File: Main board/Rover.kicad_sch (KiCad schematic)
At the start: 11 parts, among them J1 IN, J2 OUT, J3 Barrel_Jack_Switch, J4 MOTOR, J5 MOTOR, J6 MOTOR, J7 MOTOR, SW1 SW_DPDT_x2, U1 RASPBERRY_PI_4B_4GB

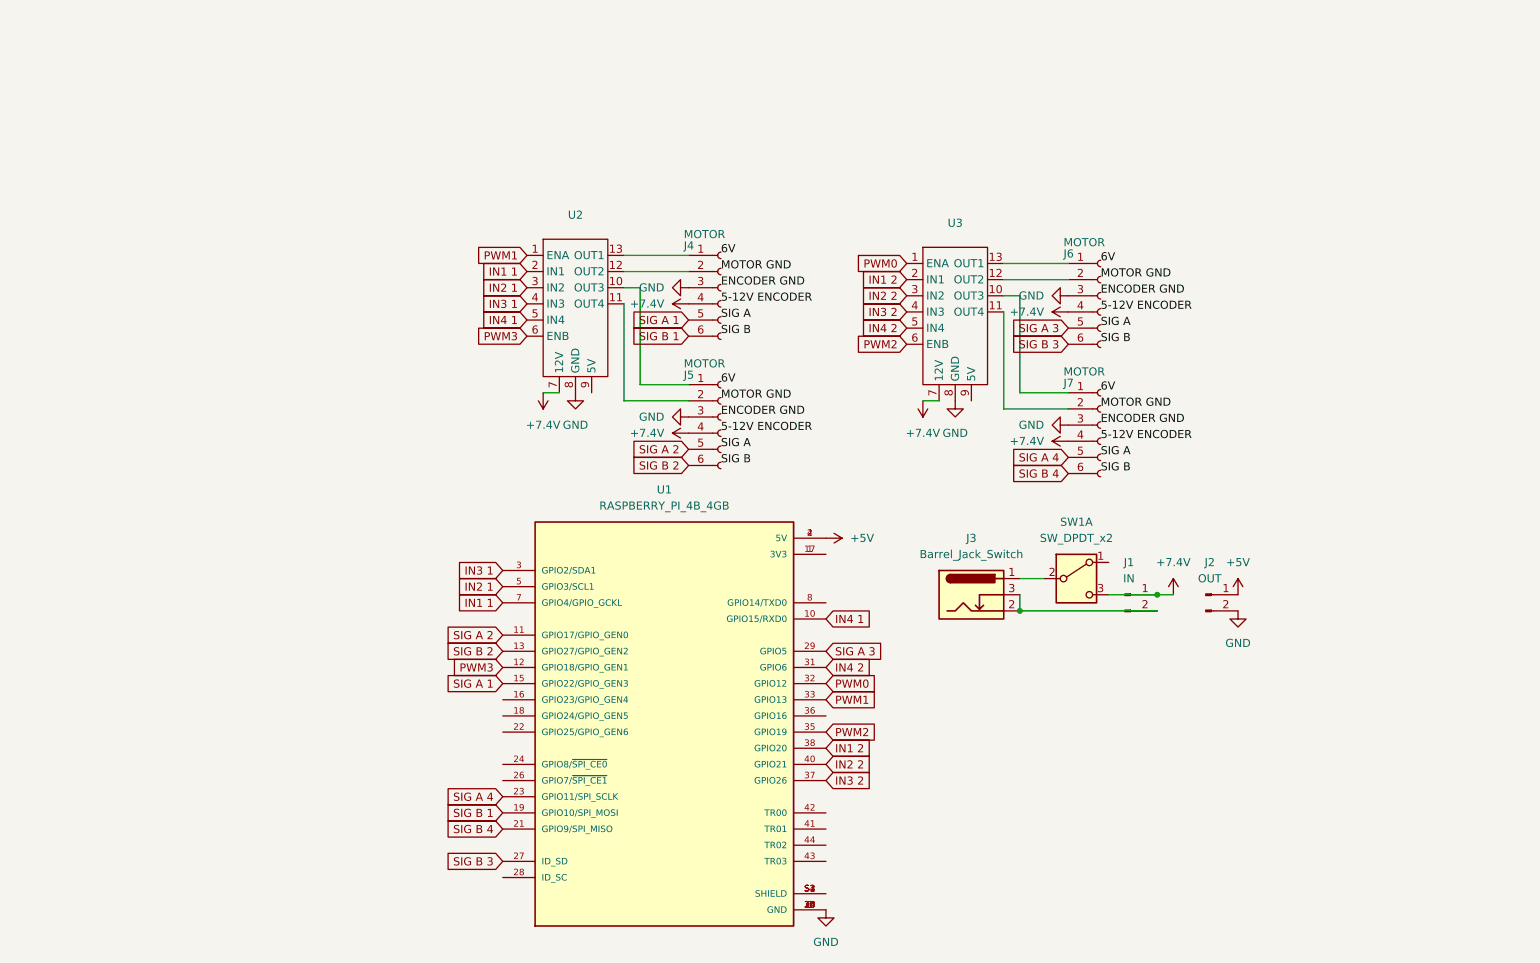
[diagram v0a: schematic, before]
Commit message: updated pcb
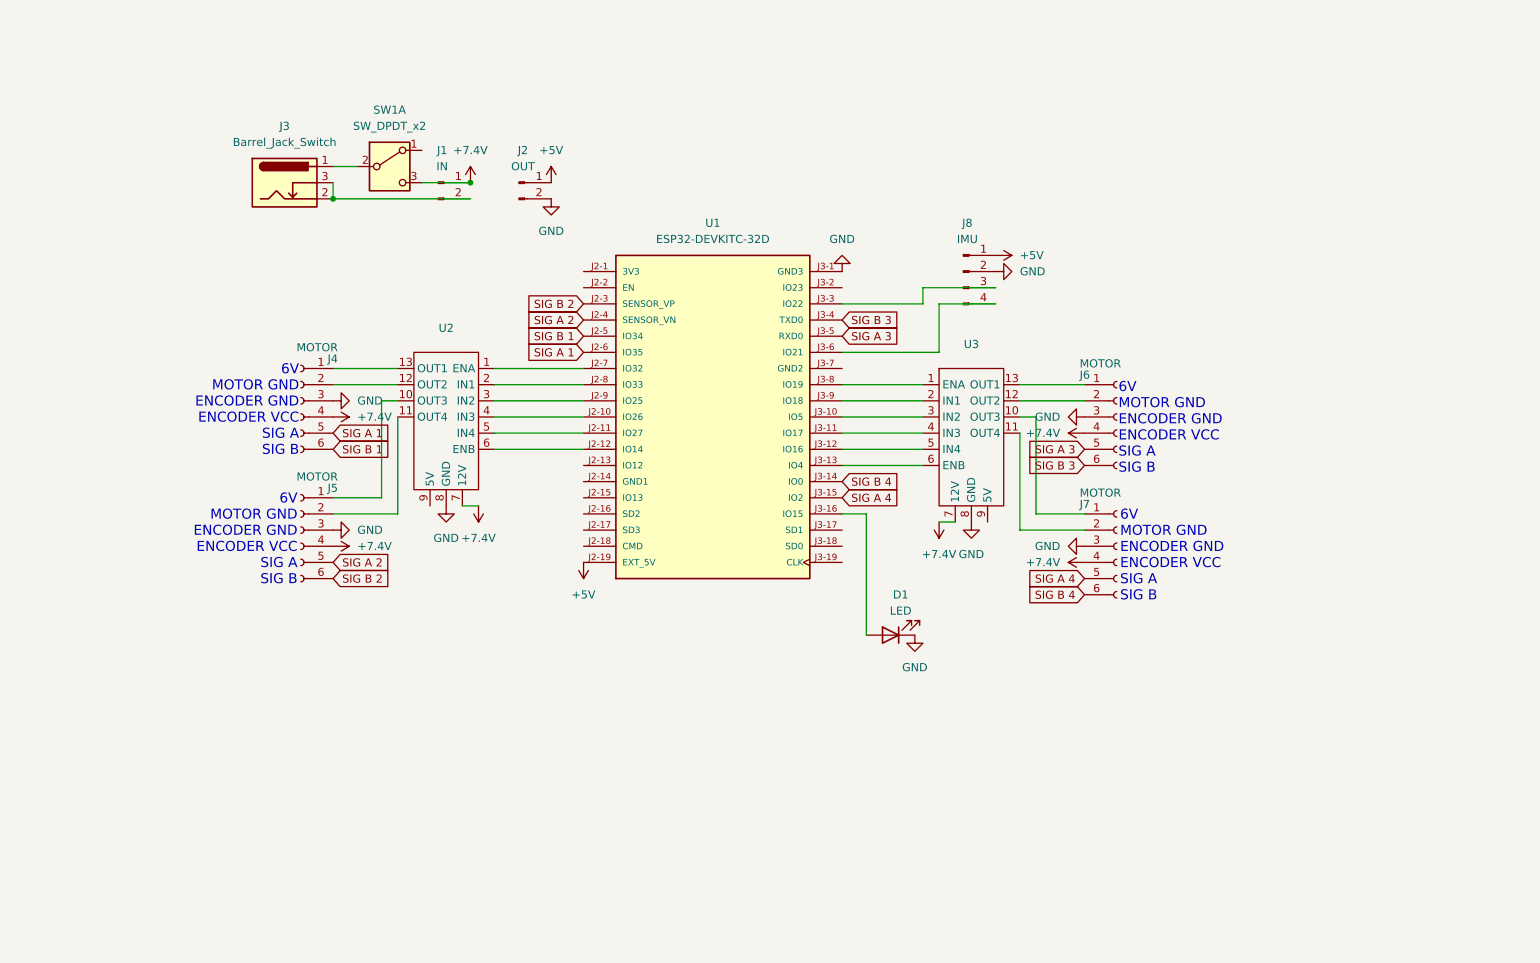
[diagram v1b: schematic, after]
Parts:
- removed U1: RASPBERRY_PI_4B_4GB, RASPBERRY_PI_4B_4GB:MODULE_RASPBERRY_PI_4B_4GB, symbol RASPBERRY_PI_4B_4GB:RASPBERRY_PI_4B_4GB
- added D1: LED, LED_THT:LED_D5.0mm_Clear, symbol Device:LED
- added J8: IMU, Connector_PinHeader_2.54mm:PinHeader_1x08_P2.54mm_Vertical, symbol Connector:Conn_01x04_Pin
- added U1: ESP32-DEVKITC-32D, Library:MODULE_ESP32-DEVKITC-32D, symbol ESP32-DEVKITC-32D:ESP32-DEVKITC-32D
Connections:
- net +5V: now also J8.1 (Pin_1), U1.J2-19 (EXT_5V)
- net GND: now also D1.1 (K), J8.2 (Pin_2), U1.J3-1 (GND3)
- net SIG A 1: now also U1.J2-6 (IO35)
- net SIG A 2: now also U1.J2-4 (SENSOR_VN)
- net SIG A 3: now also U1.J3-5 (RXD0)
- net SIG A 4: now also U1.J3-15 (IO2)
- net SIG B 1: now also U1.J2-5 (IO34)
- net SIG B 2: now also U1.J2-3 (SENSOR_VP)
- net SIG B 3: now also U1.J3-4 (TXD0)
- net SIG B 4: now also U1.J3-14 (IO0)
- net IN1 1: no longer names the net of U2.2 (IN1)
- net IN1 1: now also U1.J2-8 (IO33)
- net IN1 2: no longer names the net of U3.2 (IN1)
- net IN1 2: now also U1.J3-9 (IO18)
- net IN2 1: no longer names the net of U2.3 (IN2)
- net IN2 1: now also U1.J2-9 (IO25)
- net IN2 2: no longer names the net of U3.3 (IN2)
- net IN2 2: now also U1.J3-10 (IO5)
- net IN3 1: no longer names the net of U2.4 (IN3)
- net IN3 1: now also U1.J2-10 (IO26)
- net IN3 2: no longer names the net of U3.4 (IN3)
- net IN3 2: now also U1.J3-11 (IO17)
- net IN4 1: no longer names the net of U2.5 (IN4)
- net IN4 1: now also U1.J2-11 (IO27)
- net IN4 2: no longer names the net of U3.5 (IN4)
- net IN4 2: now also U1.J3-12 (IO16)
- net PWM0: no longer names the net of U3.1 (ENA)
- net PWM0: now also U1.J3-8 (IO19)
- net PWM1: no longer names the net of U2.1 (ENA)
- net PWM1: now also U1.J2-7 (IO32)
- net PWM2: no longer names the net of U3.6 (ENB)
- net PWM2: now also U1.J3-13 (IO4)
- net PWM3: no longer names the net of U2.6 (ENB)
- net PWM3: now also U1.J2-12 (IO14)
- new net: J8.3 (Pin_3), U1.J3-3 (IO22)
- new net: J8.4 (Pin_4), U1.J3-6 (IO21)
- new net: D1.2 (A), U1.J3-16 (IO15)
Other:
- note added: "6V MOTOR GND ENCODER GND ENCODER VCC SIG A SIG B"
- moved on the sheet: J1, J2, J3, J4, J5, J6, J7, SW1A, U2, U3

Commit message: message
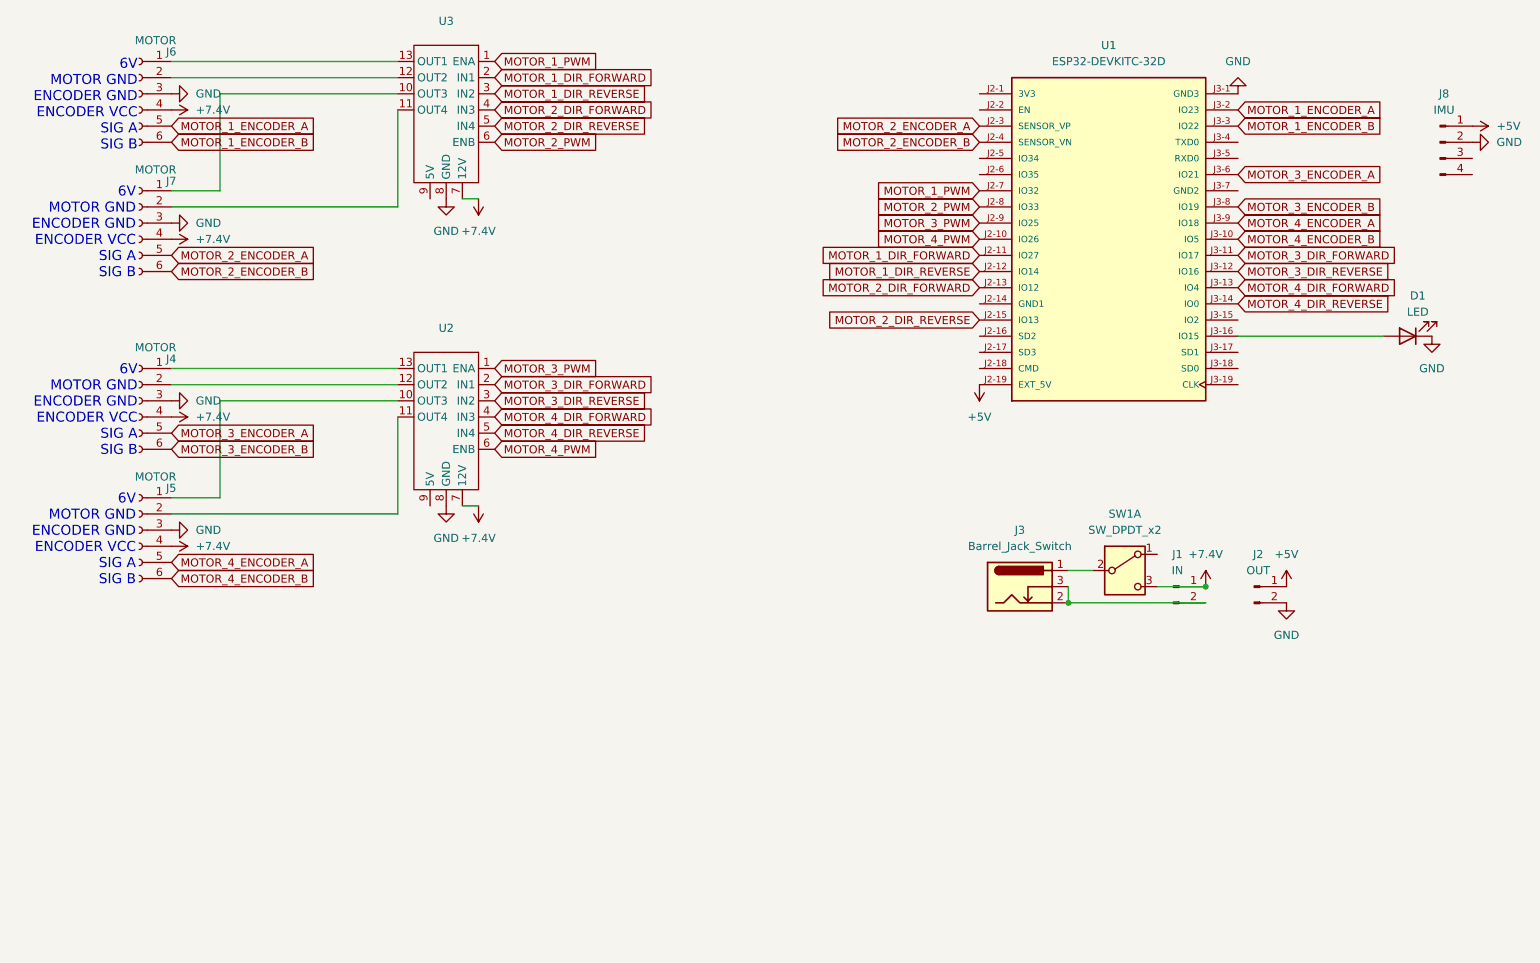
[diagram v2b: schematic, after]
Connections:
- net at J8.3 (Pin_3): no longer U1.J3-3 (IO22)
- net at J8.4 (Pin_4): no longer U1.J3-6 (IO21)
- net MOTOR_4_DIR_FORWARD: now reaches U2.4 (IN3)
- net MOTOR_4_DIR_FORWARD: now also U1.J3-13 (IO4); no longer U1.J2-10 (IO26)
- net MOTOR_1_DIR_FORWARD: now reaches U1.J2-11 (IO27)
- net MOTOR_1_DIR_FORWARD: now also U3.2 (IN1); no longer U2.5 (IN4)
- net MOTOR_1_DIR_REVERSE: now reaches U1.J2-12 (IO14)
- net MOTOR_1_DIR_REVERSE: now also U3.3 (IN2); no longer U2.6 (ENB)
- net MOTOR_2_DIR_FORWARD: now reaches U1.J2-13 (IO12)
- net MOTOR_2_DIR_FORWARD: now also U3.4 (IN3)
- net MOTOR_2_DIR_REVERSE: now reaches U1.J2-15 (IO13)
- net MOTOR_2_DIR_REVERSE: now also U3.5 (IN4)
- net MOTOR_1_PWM: now reaches U1.J2-7 (IO32)
- net MOTOR_1_PWM: now also U3.1 (ENA); no longer U2.1 (ENA)
- net MOTOR_2_PWM: now reaches U1.J2-8 (IO33)
- net MOTOR_2_PWM: now also U3.6 (ENB); no longer U2.2 (IN1)
- net MOTOR_3_DIR_REVERSE: now reaches U2.3 (IN2)
- net MOTOR_3_DIR_REVERSE: now also U1.J3-12 (IO16); no longer U1.J2-9 (IO25)
- net MOTOR_4_ENCODER_B: now reaches U1.J3-10 (IO5)
- net MOTOR_4_ENCODER_B: now also J5.6 (Pin_6); no longer U3.3 (IN2)
- net MOTOR_3_DIR_FORWARD: now reaches U1.J3-11 (IO17)
- net MOTOR_3_DIR_FORWARD: now also U2.2 (IN1); no longer U3.4 (IN3)
- net MOTOR_1_ENCODER_A: now reaches U1.J3-2 (IO23)
- net MOTOR_1_ENCODER_A: now also J6.5 (Pin_5)
- net MOTOR_3_ENCODER_B: now reaches U1.J3-8 (IO19)
- net MOTOR_3_ENCODER_B: now also J4.6 (Pin_6); no longer U3.1 (ENA)
- net MOTOR_4_ENCODER_A: now reaches U1.J3-9 (IO18)
- net MOTOR_4_ENCODER_A: now also J5.5 (Pin_5); no longer U3.2 (IN1)
- net SIG A 1: no longer names the net of U1.J2-6 (IO35)
- net SIG A 1: no longer J4.5 (Pin_5)
- net SIG A 2 renamed MOTOR_2_ENCODER_B
- net MOTOR_2_ENCODER_B: now also J7.6 (Pin_6); no longer J5.5 (Pin_5)
- net SIG A 3: no longer names the net of U1.J3-5 (RXD0)
- net SIG A 3: no longer J6.5 (Pin_5)
- net SIG A 4: no longer names the net of U1.J3-15 (IO2)
- net SIG A 4: no longer J7.5 (Pin_5)
- net SIG B 1: no longer names the net of U1.J2-5 (IO34)
- net SIG B 1: no longer J4.6 (Pin_6)
- net SIG B 2 renamed MOTOR_2_ENCODER_A
- net MOTOR_2_ENCODER_A: now also J7.5 (Pin_5); no longer J5.6 (Pin_6)
- net SIG B 3: no longer names the net of U1.J3-4 (TXD0)
- net SIG B 3: no longer J6.6 (Pin_6)
- net SIG B 4 renamed MOTOR_4_DIR_REVERSE
- net MOTOR_4_DIR_REVERSE: now also U2.5 (IN4); no longer J7.6 (Pin_6)
- new net MOTOR_1_ENCODER_B: J6.6 (Pin_6), U1.J3-3 (IO22)
- new net MOTOR_3_ENCODER_A: J4.5 (Pin_5), U1.J3-6 (IO21)
- new net MOTOR_3_PWM: U1.J2-9 (IO25), U2.1 (ENA)
- new net MOTOR_4_PWM: U1.J2-10 (IO26), U2.6 (ENB)
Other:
- moved on the sheet: D1, J1, J2, J3, J4, J5, J6, J7, J8, SW1A, U1, U3
